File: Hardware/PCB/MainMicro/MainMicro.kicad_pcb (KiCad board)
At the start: 2 copper layers, 65.8 x 81.3 mm, 56 parts, among them J1 Conn_02x05_Odd_Even, J10 Conn_01x03_Male, J11 Conn_01x05_Male, J12 Conn_01x05_Male, J2 USB_B_Mini, J3 Barrel_Jack, J4 Conn_01x05_Male, J5 Conn_01x06_Male, J6 Conn_01x06_Male, J7 Conn_01x03_Male, J8 Conn_01x03_Male, J9 Conn_01x03_Male, SW1 SW_Push, U1 AMS1117-3.3, U2 STM32F091RCTx, U3 FT232RL, U4 MAX7375AXR805, U5 SN74AVC8T245PW

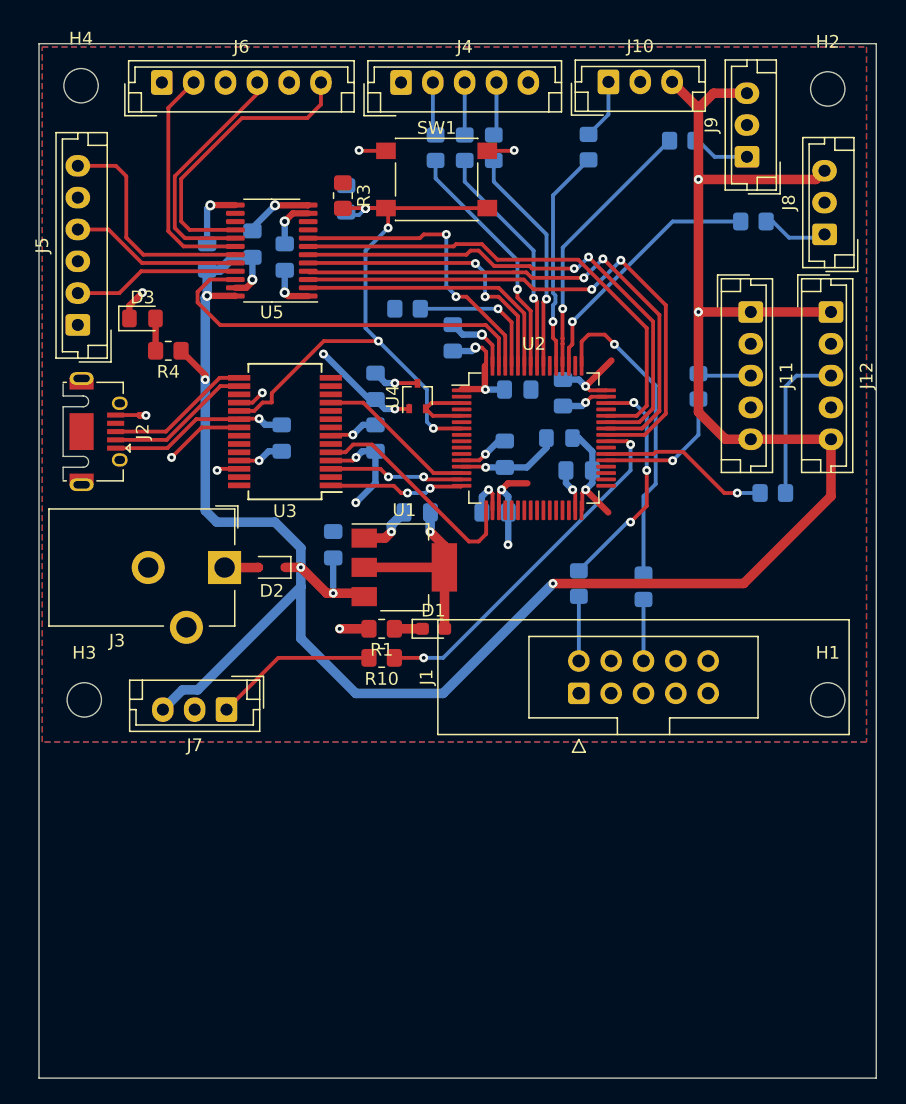
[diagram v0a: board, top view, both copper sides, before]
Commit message: PCB passing DRC
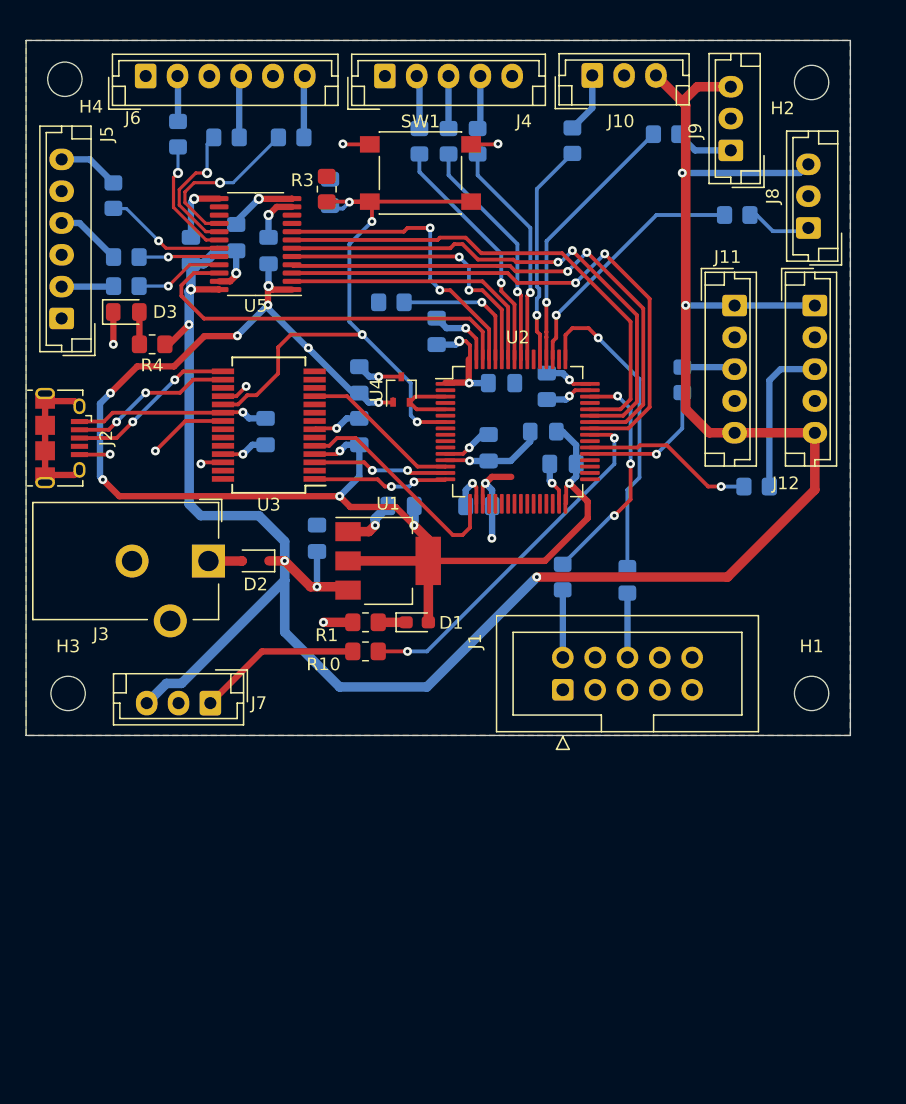
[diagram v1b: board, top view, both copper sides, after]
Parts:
- added R16: 10, Resistor_SMD:R_0805_2012Metric_Pad1.20x1.40mm_HandSolder, B.Cu at (155.2, 85.3)
- added R17: 10, Resistor_SMD:R_0805_2012Metric_Pad1.20x1.40mm_HandSolder, B.Cu at (155.2, 83.1)
- added R18: 10, Resistor_SMD:R_0805_2012Metric_Pad1.20x1.40mm_HandSolder, B.Cu at (154.2, 78.2)
- added R19: 10, Resistor_SMD:R_0805_2012Metric_Pad1.20x1.40mm_HandSolder, B.Cu at (159.3, 73.4)
- added R20: 10, Resistor_SMD:R_0805_2012Metric_Pad1.20x1.40mm_HandSolder, B.Cu at (163.1, 73.7)
- added R21: 10, Resistor_SMD:R_0805_2012Metric_Pad1.20x1.40mm_HandSolder, B.Cu at (168.1, 73.7)
- J2: footprint Connector_USB:USB_Micro-AB_Molex_47590-0001 -> Connector_USB:USB_Micro-B_Amphenol_10118194_Horizontal
- moved J1 4.75 mm to (194.6, 114.5)
- moved J2 1.65 mm to (150.1, 97.3)
- moved C11 1.37 mm to (173.5, 92.7)
- moved C15 1.37 mm to (160.3, 82.5)
- moved C3 1.37 mm to (171.2, 78.0)
- moved C9 1.37 mm to (183.7, 98.0)
- moved H4 1.37 mm to (150.4, 69.1)
- moved J10 1.37 mm to (191.8, 68.8)
- moved J11 1.37 mm to (203.0, 86.9)
- moved J12 1.37 mm to (209.3, 86.9)
- moved R4 1.37 mm to (157.2, 89.9)
- moved SW1 1.37 mm to (178.3, 76.5)
- moved U4 1.37 mm to (176.8, 93.5)
- moved C10 1.37 mm to (166.1, 96.8)
- moved C12 1.37 mm to (173.5, 96.8)
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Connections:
- U5 pad 16: /EN2+ -> Net-(U5-Pad16)
- U5 pad 17: /DIR2+ -> Net-(U5-Pad17)
- U5 pad 18: /PUL2+ -> Net-(U5-Pad18)
- U5 pad 19: /EN1+ -> Net-(U5-Pad19)
- U5 pad 20: /DIR1+ -> Net-(U5-Pad20)
- U5 pad 21: /PUL1+ -> Net-(U5-Pad21)
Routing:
- net +3V3: track 71.0 -> 136.7 mm, vias 12 -> 16
- net /EN2+: track 23.0 -> 4.85 mm
- net /PUL2+: track 18.3 -> 3.59 mm
- net /DIR2+: track 19.2 -> 4.89 mm
- net Net-(U5-Pad16): track 0.00 -> 13.3 mm, vias 0 -> 1
- net /EN1+: track 18.1 -> 4.83 mm
- net unconnected-(J2-Pad6): track 0.00 -> 11.5 mm
- net Net-(U5-Pad17): track 0.00 -> 11.0 mm, vias 0 -> 1
- net Net-(U5-Pad19): track 0.00 -> 9.61 mm, vias 0 -> 1
- net Net-(U5-Pad18): track 0.00 -> 9.55 mm, vias 0 -> 1
- net /PUL1+: track 13.1 -> 4.10 mm
- net /DIR1+: track 13.5 -> 5.19 mm
- net Net-(U5-Pad21): track 0.00 -> 6.99 mm, vias 0 -> 1
- net Net-(U5-Pad20): track 0.00 -> 6.31 mm, vias 0 -> 1
- net /USB_D+: track 11.5 -> 13.4 mm, vias 0 -> 2
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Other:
- board size 65.8 x 81.3 mm -> 64.8 x 54.6 mm
